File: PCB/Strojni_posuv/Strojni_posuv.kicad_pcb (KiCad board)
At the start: 2 copper layers, 170 x 80 mm, 115 parts, among them IC1 TB6600HG, J1 Conn_01x20_Pin, J10 Button_right_B, J2 Button_power_A, J5 POWER, J6 Button_power_B, J7 Button_left_A, J8 Button_left_B, J9 Button_right_A, Q1 BSS138, Q2 BSS138, Q3 BSS138, Q4 BSS138, Q5 BSS138, Q6 BSS138, Q7 BC847, SW1 SW_DPST_x2, SW2 SW_DPST_x2, SW3 SW_DPST_x2, U1 STM32F103RBTx, U3 6N137, U5 6N137, U6 PC817, U7 74HC14, U8 TPS62822DLC, Y1 16MHz

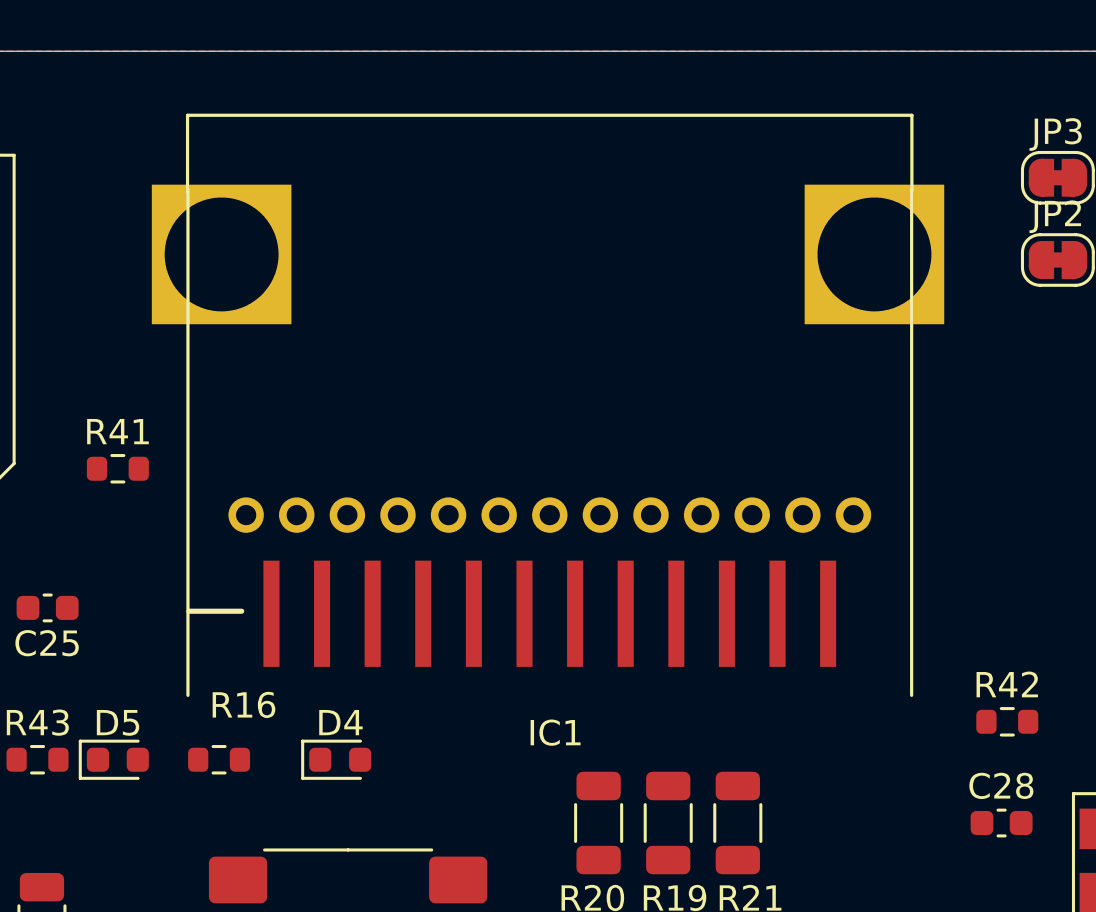
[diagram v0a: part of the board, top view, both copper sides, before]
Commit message: New materials + Schuzka
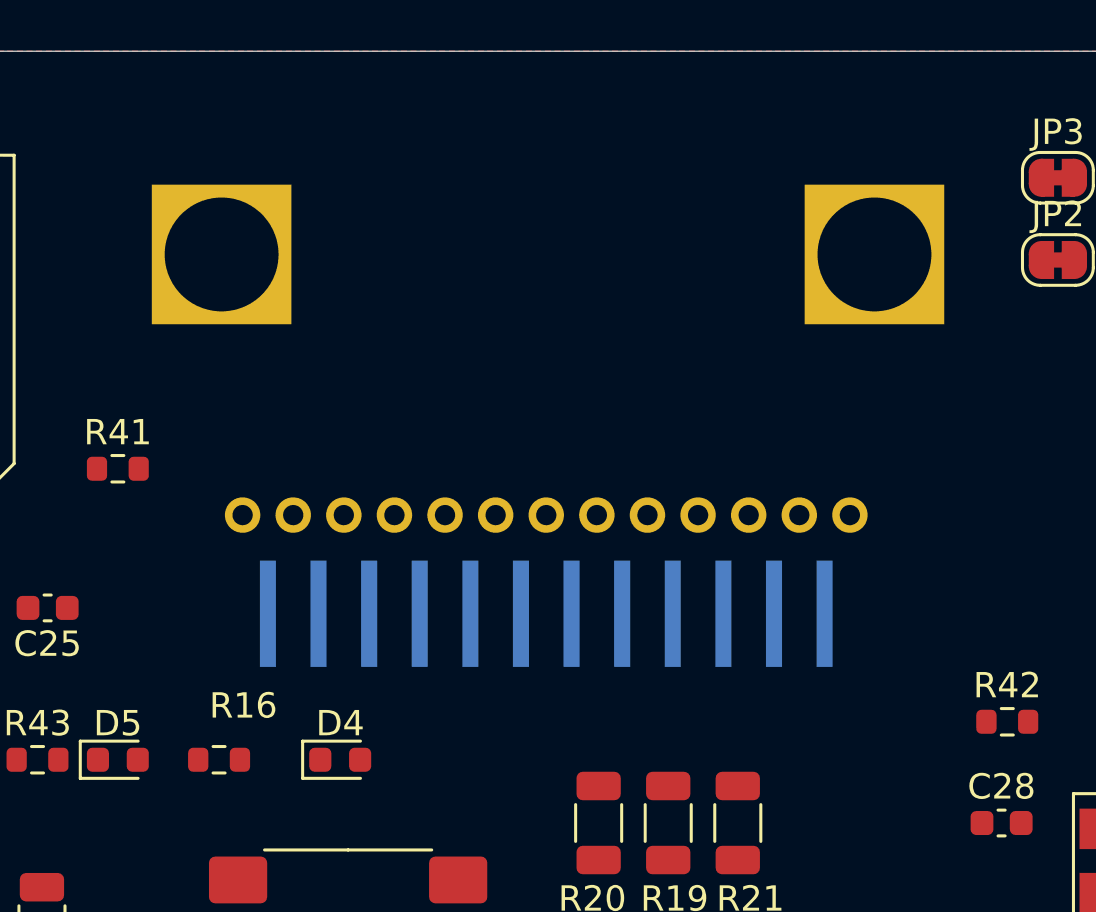
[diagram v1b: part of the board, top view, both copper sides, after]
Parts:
- IC1: moved to B.Cu
- moved IC1 2.14 mm to (98.9, 51.0), turned to 0 degrees
